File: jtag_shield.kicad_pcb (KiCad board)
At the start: 2 copper layers, 100 x 68.5 mm, 8 parts, among them J1 AVR-JTAG-10, J2 AVR-ISP-6, Q1 BF245A

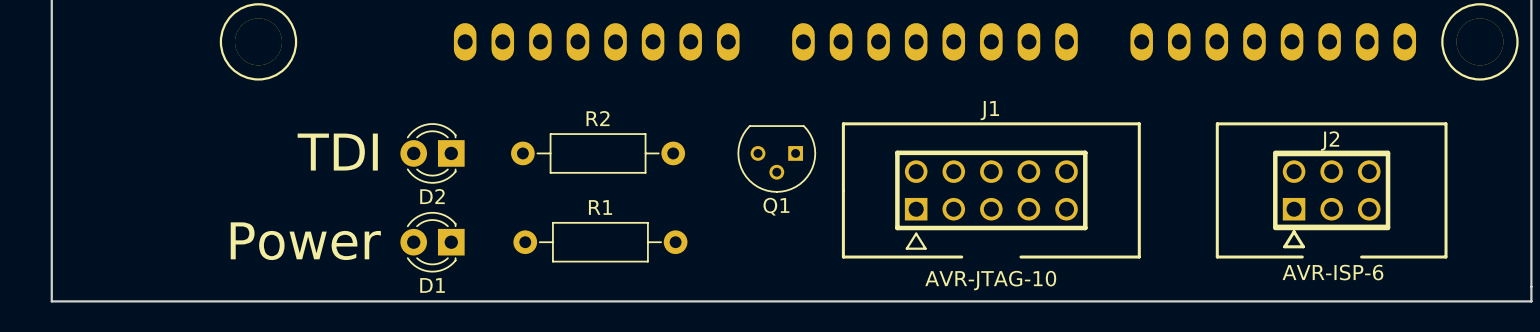
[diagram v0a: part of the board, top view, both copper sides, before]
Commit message: Updated with changes from Magnus
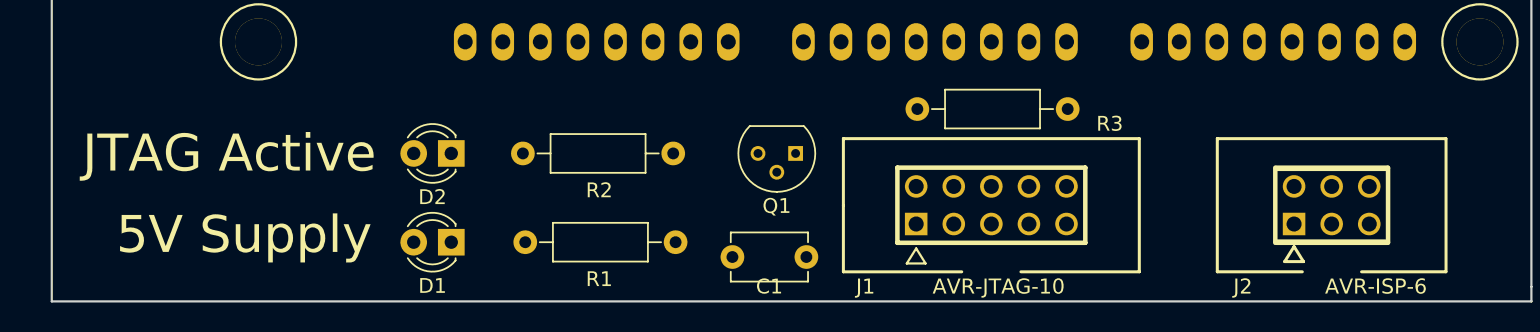
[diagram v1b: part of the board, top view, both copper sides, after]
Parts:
- added C1: 100n, Capacitors_THT:C_Disc_D5.1mm_W3.2mm_P5.00mm, F.Cu at (101.0, 112.0)
- added R3: 47k, Resistors_THT:R_Axial_DIN0207_L6.3mm_D2.5mm_P10.16mm_Horizontal, F.Cu at (108.5, 102.0)
- moved J1 1.00 mm to (113.5, 108.5)
- moved J2 1.00 mm to (136.5, 108.5)
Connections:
- Q1 pad 1: /TDI -> Net-(Q1-Pad1)
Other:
- board text added: "5V Supply"
- board text added: "JTAG Active"
- board text removed: "Power"
- board text removed: "TDI"
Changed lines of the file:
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@@
 (kicad_pcb (version 4) (host pcbnew 4.0.6)
   (general
-    (links 33)
-    (no_connects 33)
+    (links 36)
+    (no_connects 36)
     (area 49.924999 46.424999 150.075001 115.075001)
     (thickness 1.6)
@@
     (tracks 0)
     (zones 0)
-    (modules 8)
-    (nets 14)
+    (modules 10)
+    (nets 15)
   )
   (page A4)
@@
     (47 F.CrtYd user)
     (48 B.Fab user)
-    (49 F.Fab user)
+    (49 F.Fab user hide)
   )
   (setup
@@
     (aux_axis_origin 0 0)
     (grid_origin 50 100)
-    (visible_elements FFFFFF7F)
+    (visible_elements 7FFFFFFF)
     (pcbplotparams
       (layerselection 0x00030_80000001)
@@
   (net 12 /SCK)
   (net 13 /MOSI)
+  (net 14 "Net-(Q1-Pad1)")
   (net_class Default "This is the default net class."
     (clearance 0.2032)
@@
     (add_net "Net-(D1-Pad1)")
     (add_net "Net-(D2-Pad1)")
+    (add_net "Net-(Q1-Pad1)")
     (add_net "Net-(Q1-Pad3)")
   )
@@
       (net 2 "Net-(Q1-Pad3)"))
     (pad 1 thru_hole rect (at 0 0 270) (size 1 1) (drill 0.6) (layers *.Cu *.Mask)
-      (net 3 /TDI))
+      (net 14 "Net-(Q1-Pad1)"))
     (model TO_SOT_Packages_THT.3dshapes/TO-92_Molded_Narrow.wrl
       (at (xyz 0.05 0 0))
@@
       (effects (font (size 1 1) (thickness 0.15)))
     )
-    (fp_text value LED (at 1.27 2.96 180) (layer F.Fab)
+    (fp_text value LED (at 1 1.5 180) (layer F.Fab)
       (effects (font (size 1 1) (thickness 0.15)))
     )
@@
       (effects (font (size 1 1) (thickness 0.15)))
     )
-    (fp_text value LED (at 1.27 2.96 180) (layer F.Fab)
+    (fp_text value LED (at 1 1.5 180) (layer F.Fab)
       (effects (font (size 1 1) (thickness 0.15)))
     )
@@
     (descr "Resistor, Axial_DIN0207 series, Axial, Horizontal, pin pitch=10.16mm, 0.25W = 1/4W, length*diameter=6.3*2.5mm^2, http://cdn-reichelt.de/documents/datenblatt/B400/1_4W%23YAG.pdf")
     (tags "Resistor Axial_DIN0207 series Axial Horizontal pin pitch 10.16mm 0.25W = 1/4W length 6.3mm diameter 2.5mm")
-    (fp_text reference R1 (at 5.08 -2.31) (layer F.SilkS)
-      (effects (font (size 1 1) (thickness 0.15)))
-    )
-    (fp_text value 470R (at 5.08 2.31) (layer F.Fab)
+    (fp_text reference R1 (at 5 2.5) (layer F.SilkS)
+      (effects (font (size 1 1) (thickness 0.15)))
+    )
+    (fp_text value 470R (at 5 0) (layer F.Fab)
       (effects (font (size 1 1) (thickness 0.15)))
     )
@@
     (descr "Resistor, Axial_DIN0207 series, Axial, Horizontal, pin pitch=10.16mm, 0.25W = 1/4W, length*diameter=6.3*2.5mm^2, http://cdn-reichelt.de/documents/datenblatt/B400/1_4W%23YAG.pdf")
     (tags "Resistor Axial_DIN0207 series Axial Horizontal pin pitch 10.16mm 0.25W = 1/4W length 6.3mm diameter 2.5mm")
-    (fp_text reference R2 (at 5.08 -2.31) (layer F.SilkS)
-      (effects (font (size 1 1) (thickness 0.15)))
-    )
-    (fp_text value 470R (at 5.08 2.31) (layer F.Fab)
+    (fp_text reference R2 (at 5.16 2.5) (layer F.SilkS)
+      (effects (font (size 1 1) (thickness 0.15)))
+    )
+    (fp_text value 470R (at 5.16 0) (layer F.Fab)
       (effects (font (size 1 1) (thickness 0.15)))
     )
@@
   )
   (module rmc_modules:PIN_ARRAY_5x2_RMC (layer F.Cu)
-    (at 113.5 107.5)
+    (at 113.5 108.5)
     (descr "Double rangee de contacts 2 x 5 pins")
     (tags CONN)
-    (fp_text reference J1 (at 0 -5.4991) (layer F.SilkS)
+    (fp_text reference J1 (at -8.5 5.5) (layer F.SilkS)
       (effects (font (size 1.016 1.016) (thickness 0.2032)))
     )
-    (fp_text value AVR-JTAG-10 (at 0 6) (layer F.SilkS)
+    (fp_text value AVR-JTAG-10 (at 0.5 5.5) (layer F.SilkS)
       (effects (font (size 1.016 1.016) (thickness 0.2032)))
     )
@@
   )
   (module rmc_modules:pin_array_3x2_RMC (layer F.Cu)
-    (at 136.5 107.5)
+    (at 136.5 108.5)
     (descr "Double rangee de contacts 2 x 4 pins")
     (tags CONN)
-    (fp_text reference J2 (at 0 -3.429) (layer F.SilkS)
+    (fp_text reference J2 (at -6 5.5) (layer F.SilkS)
       (effects (font (size 1.016 1.016) (thickness 0.2032)))
     )
-    (fp_text value AVR-ISP-6 (at 0.127 5.588) (layer F.SilkS)
+    (fp_text value AVR-ISP-6 (at 3 5.5) (layer F.SilkS)
       (effects (font (size 1.016 1.016) (thickness 0.2032)))
     )
@@
       (net 8 +5V))
   )
+  (module Capacitors_THT:C_Disc_D5.1mm_W3.2mm_P5.00mm (layer F.Cu)
+    (at 101 112 180)
+    (descr "C, Disc series, Radial, pin pitch=5.00mm, , diameter*width=5.1*3.2mm^2, Capacitor, http://www.vishay.com/docs/45233/krseries.pdf")
+    (tags "C Disc series Radial pin pitch 5.00mm  diameter 5.1mm width 3.2mm Capacitor")
+    (fp_text reference C1 (at 2.5 -2 180) (layer F.SilkS)
+      (effects (font (size 1 1) (thickness 0.15)))
+    )
+    (fp_text value 100n (at 2.5 0.5 180) (layer F.Fab)
+      (effects (font (size 1 1) (thickness 0.15)))
+    )
+    (fp_line (start -0.05 -1.6) (end -0.05 1.6) (layer F.Fab) (width 0.1))
+    (fp_line (start -0.05 1.6) (end 5.05 1.6) (layer F.Fab) (width 0.1))
+    (fp_line (start 5.05 1.6) (end 5.05 -1.6) (layer F.Fab) (width 0.1))
+    (fp_line (start 5.05 -1.6) (end -0.05 -1.6) (layer F.Fab) (width 0.1))
+    (fp_line (start -0.11 -1.66) (end 5.11 -1.66) (layer F.SilkS) (width 0.12))
+    (fp_line (start -0.11 1.66) (end 5.11 1.66) (layer F.SilkS) (width 0.12))
+    (fp_line (start -0.11 -1.66) (end -0.11 -0.996) (layer F.SilkS) (width 0.12))
+    (fp_line (start -0.11 0.996) (end -0.11 1.66) (layer F.SilkS) (width 0.12))
+    (fp_line (start 5.11 -1.66) (end 5.11 -0.996) (layer F.SilkS) (width 0.12))
+    (fp_line (start 5.11 0.996) (end 5.11 1.66) (layer F.SilkS) (width 0.12))
+    (fp_line (start -1.05 -1.95) (end -1.05 1.95) (layer F.CrtYd) (width 0.05))
+    (fp_line (start -1.05 1.95) (end 6.05 1.95) (layer F.CrtYd) (width 0.05))
+    (fp_line (start 6.05 1.95) (end 6.05 -1.95) (layer F.CrtYd) (width 0.05))
+    (fp_line (start 6.05 -1.95) (end -1.05 -1.95) (layer F.CrtYd) (width 0.05))
+    (pad 1 thru_hole circle (at 0 0 180) (size 1.6 1.6) (drill 0.8) (layers *.Cu *.Mask)
+      (net 8 +5V))
+    (pad 2 thru_hole circle (at 5 0 180) (size 1.6 1.6) (drill 0.8) (layers *.Cu *.Mask)
+      (net 1 GND))
+    (model Capacitors_THT.3dshapes/C_Disc_D5.1mm_W3.2mm_P5.00mm.wrl
+      (at (xyz 0 0 0))
+      (scale (xyz 0.393701 0.393701 0.393701))
+      (rotate (xyz 0 0 0))
+    )
+  )
+  (module Resistors_THT:R_Axial_DIN0207_L6.3mm_D2.5mm_P10.16mm_Horizontal (layer F.Cu)
+    (at 108.5 102)
+    (descr "Resistor, Axial_DIN0207 series, Axial, Horizontal, pin pitch=10.16mm, 0.25W = 1/4W, length*diameter=6.3*2.5mm^2, http://cdn-reichelt.de/documents/datenblatt/B400/1_4W%23YAG.pdf")
+    (tags "Resistor Axial_DIN0207 series Axial Horizontal pin pitch 10.16mm 0.25W = 1/4W length 6.3mm diameter 2.5mm")
+    (fp_text reference R3 (at 13 1) (layer F.SilkS)
+      (effects (font (size 1 1) (thickness 0.15)))
+    )
+    (fp_text value 47k (at 13 -0.5) (layer F.Fab)
+      (effects (font (size 1 1) (thickness 0.15)))
+    )
+    (fp_line (start 1.93 -1.25) (end 1.93 1.25) (layer F.Fab) (width 0.1))
+    (fp_line (start 1.93 1.25) (end 8.23 1.25) (layer F.Fab) (width 0.1))
+    (fp_line (start 8.23 1.25) (end 8.23 -1.25) (layer F.Fab) (width 0.1))
+    (fp_line (start 8.23 -1.25) (end 1.93 -1.25) (layer F.Fab) (width 0.1))
+    (fp_line (start 0 0) (end 1.93 0) (layer F.Fab) (width 0.1))
+    (fp_line (start 10.16 0) (end 8.23 0) (layer F.Fab) (width 0.1))
+    (fp_line (start 1.87 -1.31) (end 1.87 1.31) (layer F.SilkS) (width 0.12))
+    (fp_line (start 1.87 1.31) (end 8.29 1.31) (layer F.SilkS) (width 0.12))
+    (fp_line (start 8.29 1.31) (end 8.29 -1.31) (layer F.SilkS) (width 0.12))
+    (fp_line (start 8.29 -1.31) (end 1.87 -1.31) (layer F.SilkS) (width 0.12))
+    (fp_line (start 0.98 0) (end 1.87 0) (layer F.SilkS) (width 0.12))
+    (fp_line (start 9.18 0) (end 8.29 0) (layer F.SilkS) (width 0.12))
+    (fp_line (start -1.05 -1.6) (end -1.05 1.6) (layer F.CrtYd) (width 0.05))
+    (fp_line (start -1.05 1.6) (end 11.25 1.6) (layer F.CrtYd) (width 0.05))
+    (fp_line (start 11.25 1.6) (end 11.25 -1.6) (layer F.CrtYd) (width 0.05))
+    (fp_line (start 11.25 -1.6) (end -1.05 -1.6) (layer F.CrtYd) (width 0.05))
+    (pad 1 thru_hole circle (at 0 0) (size 1.6 1.6) (drill 0.8) (layers *.Cu *.Mask)
+      (net 14 "Net-(Q1-Pad1)"))
+    (pad 2 thru_hole oval (at 10.16 0) (size 1.6 1.6) (drill 0.8) (layers *.Cu *.Mask)
+      (net 3 /TDI))
+    (model Resistors_THT.3dshapes/R_Axial_DIN0207_L6.3mm_D2.5mm_P10.16mm_Horizontal.wrl
+      (at (xyz 0 0 0))
+      (scale (xyz 0.393701 0.393701 0.393701))
+      (rotate (xyz 0 0 0))
+    )
+  )
   (gr_line (start 50 115) (end 50 46.5) (angle 90) (layer Edge.Cuts) (width 0.15))
   (gr_line (start 150 115) (end 50 115) (angle 90) (layer Edge.Cuts) (width 0.15))
@@
   (gr_line (start 150 46.5) (end 150 114) (angle 90) (layer Edge.Cuts) (width 0.15))
   (gr_line (start 50 46.5) (end 150 46.5) (angle 90) (layer Edge.Cuts) (width 0.15))
-  (gr_text TDI (at 69.5 105) (layer F.SilkS)
+  (gr_text "JTAG Active" (at 62 105) (layer F.SilkS)
     (effects (font (size 2.5 2.5) (thickness 0.3)))
   )
-  (gr_text Power (at 67 111) (layer F.SilkS)
+  (gr_text "5V Supply" (at 63 110.5) (layer F.SilkS)
     (effects (font (size 2.5 2.5) (thickness 0.3)))
   )
